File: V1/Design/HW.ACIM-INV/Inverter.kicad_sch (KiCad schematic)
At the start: 57 parts, among them J3 MOTOR, M1 560V/1.75kA, M2 560V/1.75kA, M3 560V/1.75kA, Q1 20V/1A, U1 IPM 600V/15A, U15 I=±10A, U16 I=±10A, U20 CMP-1CH, U3 DIGI ISO, U5 DIGI ISO, U9 DIGI ISO

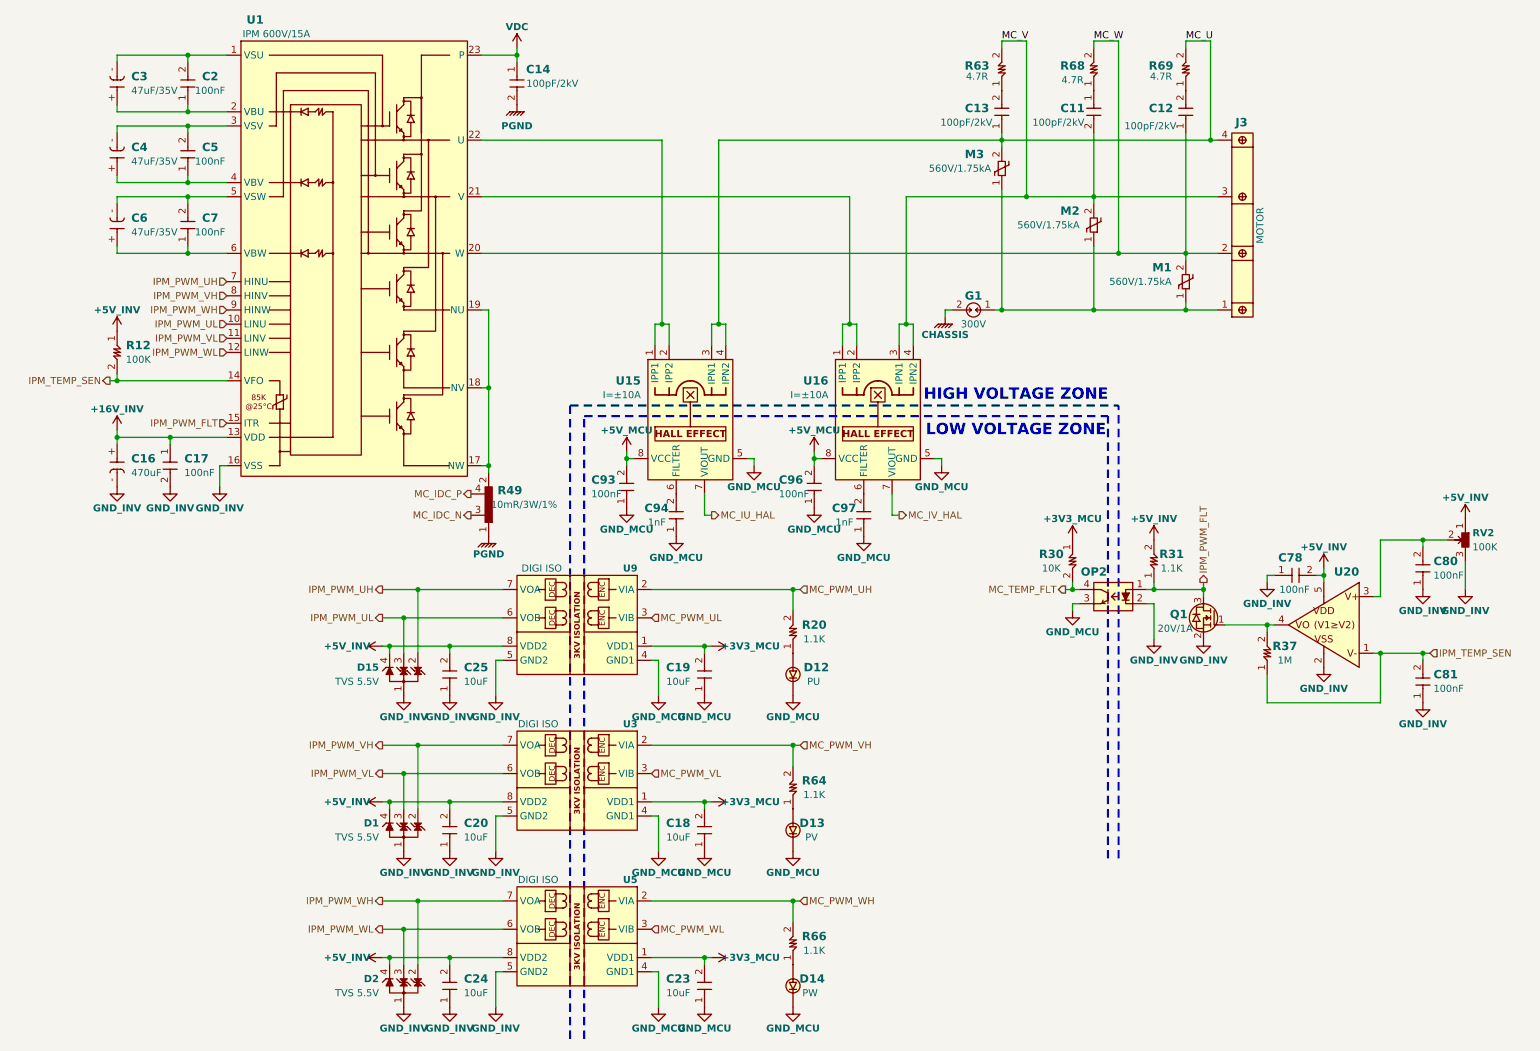
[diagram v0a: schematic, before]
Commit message: V1 schematic update 16
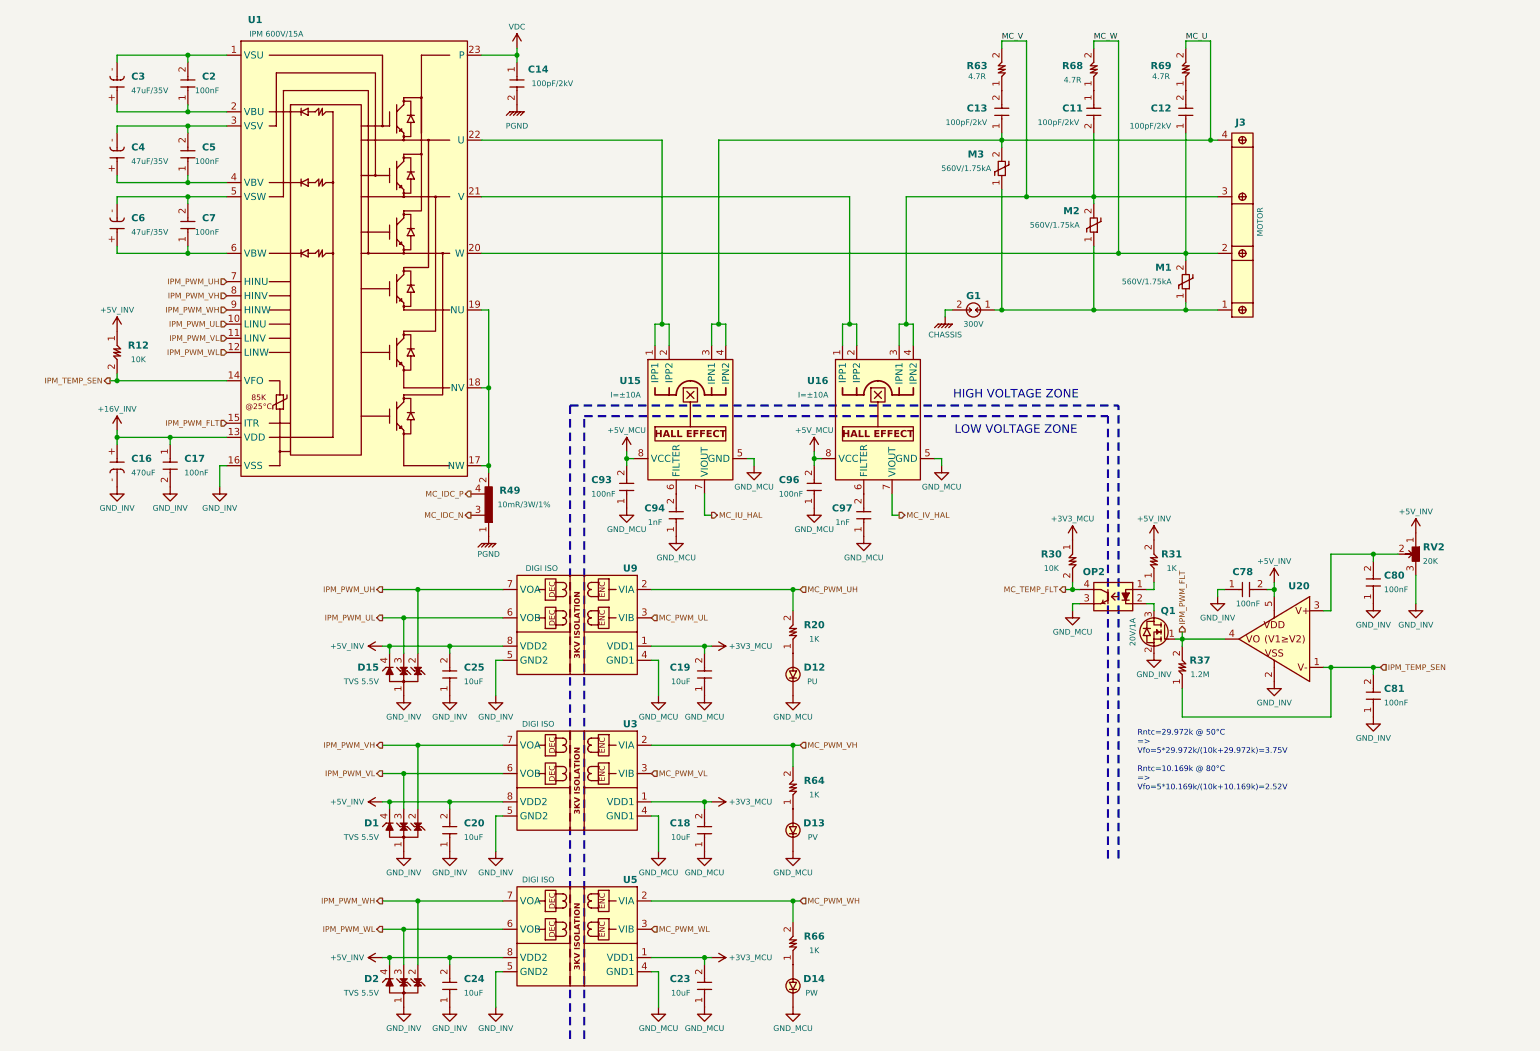
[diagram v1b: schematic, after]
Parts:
- C78, C80, C81: Checked OK -> (none); Unit Price 0.0146 -> (none)
- Q1: Checked OK -> (none); Unit Price 0.148 -> (none)
- R12: value 100K -> 10K; MFT YAGEO -> (none); MNP RC0603FR-07100KL -> (none)
- R20, R31, R64, R66: value 1.1K -> 1K; MFT YAGEO -> (none); MNP AC0603FR-071K1L -> (none)
- R30: MFT YAGEO -> (none); MNP RC0603FR-07100KL -> (none)
- R37: value 1M -> 1.2M; footprint SAMPI:RES1206 -> SAMPI:RES0603; Checked OK -> (none); MFT Walsin -> (none); MNP WR12X105 JTL -> (none); Unit Price 0.02 -> (none)
- RV2: value 100K -> 20K; MNP TC33X-2-104E -> TC33X-2-203E
- U20: Checked OK -> (none); Unit Price 0.36 -> (none)
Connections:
- net GND_INV: no longer OP2.2 (K)
- net IPM_PWM_FLT: now also Q1.1 (G), R37.2, U20.4 (VOUT); no longer OP2.1 (A), Q1.3 (D), R31.1
- new net: OP2.1 (A), R31.1
- new net: OP2.2 (K), Q1.3 (D)
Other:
- moved on the sheet: C78, C80, C81, Q1, R37, RV2, U20
